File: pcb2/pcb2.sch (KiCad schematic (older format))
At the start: 3 parts

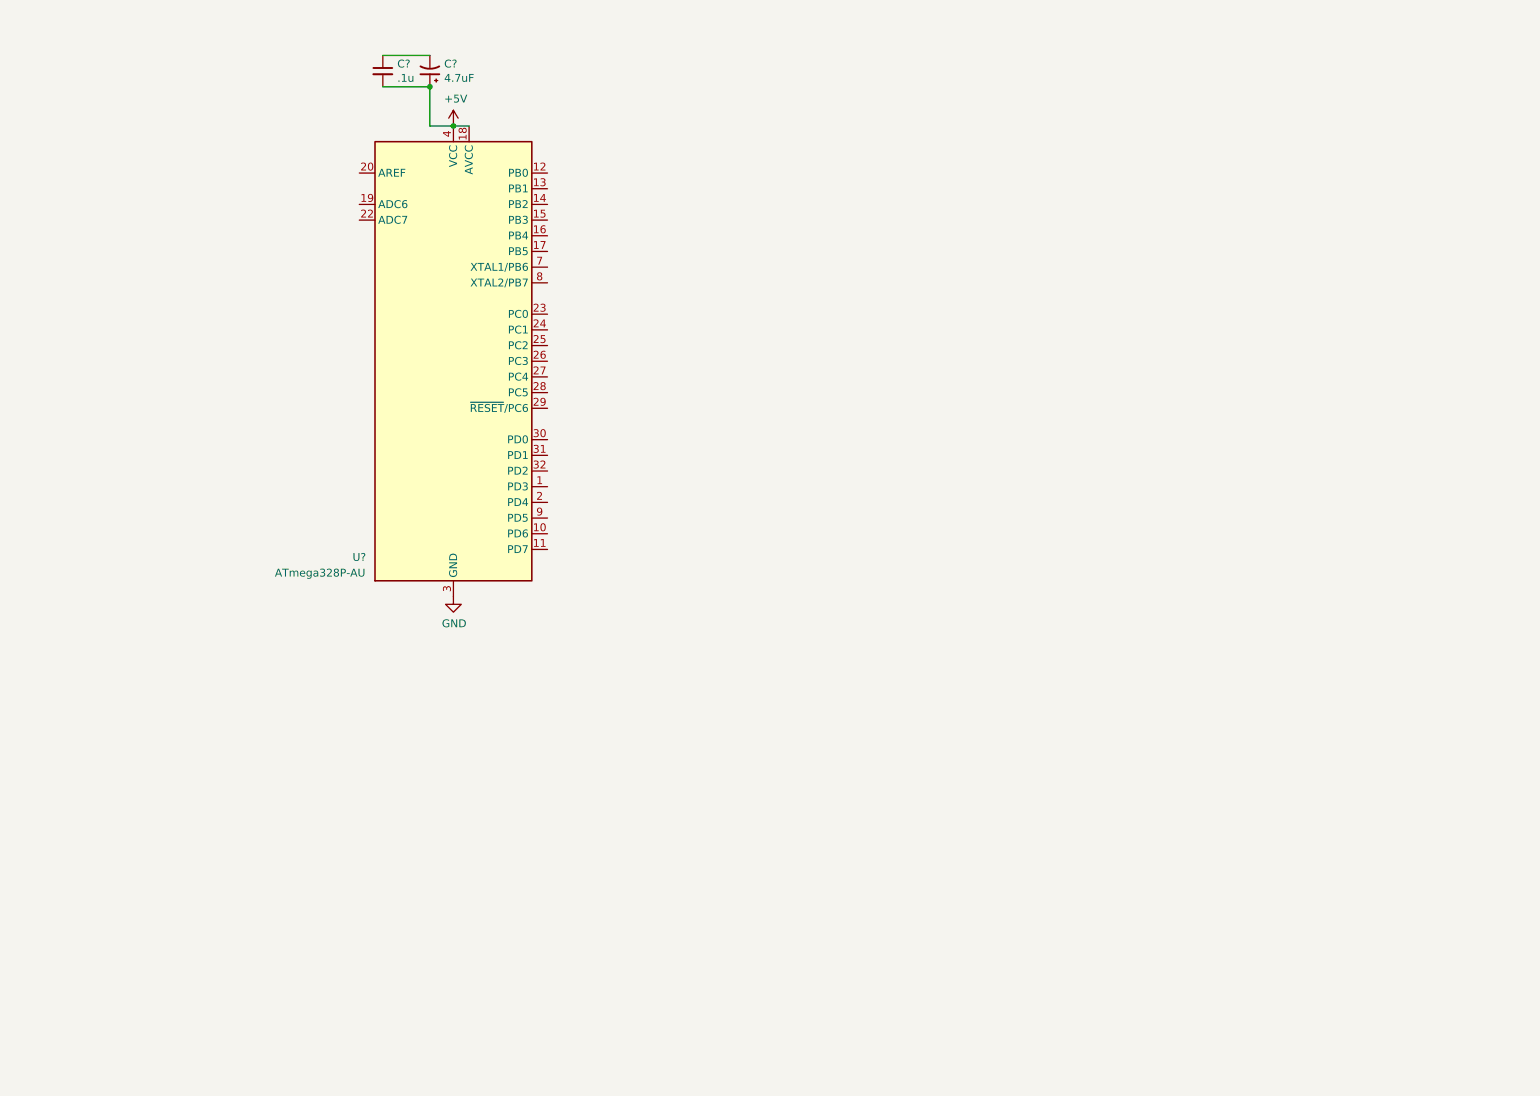
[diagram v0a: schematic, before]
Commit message: second pcb design
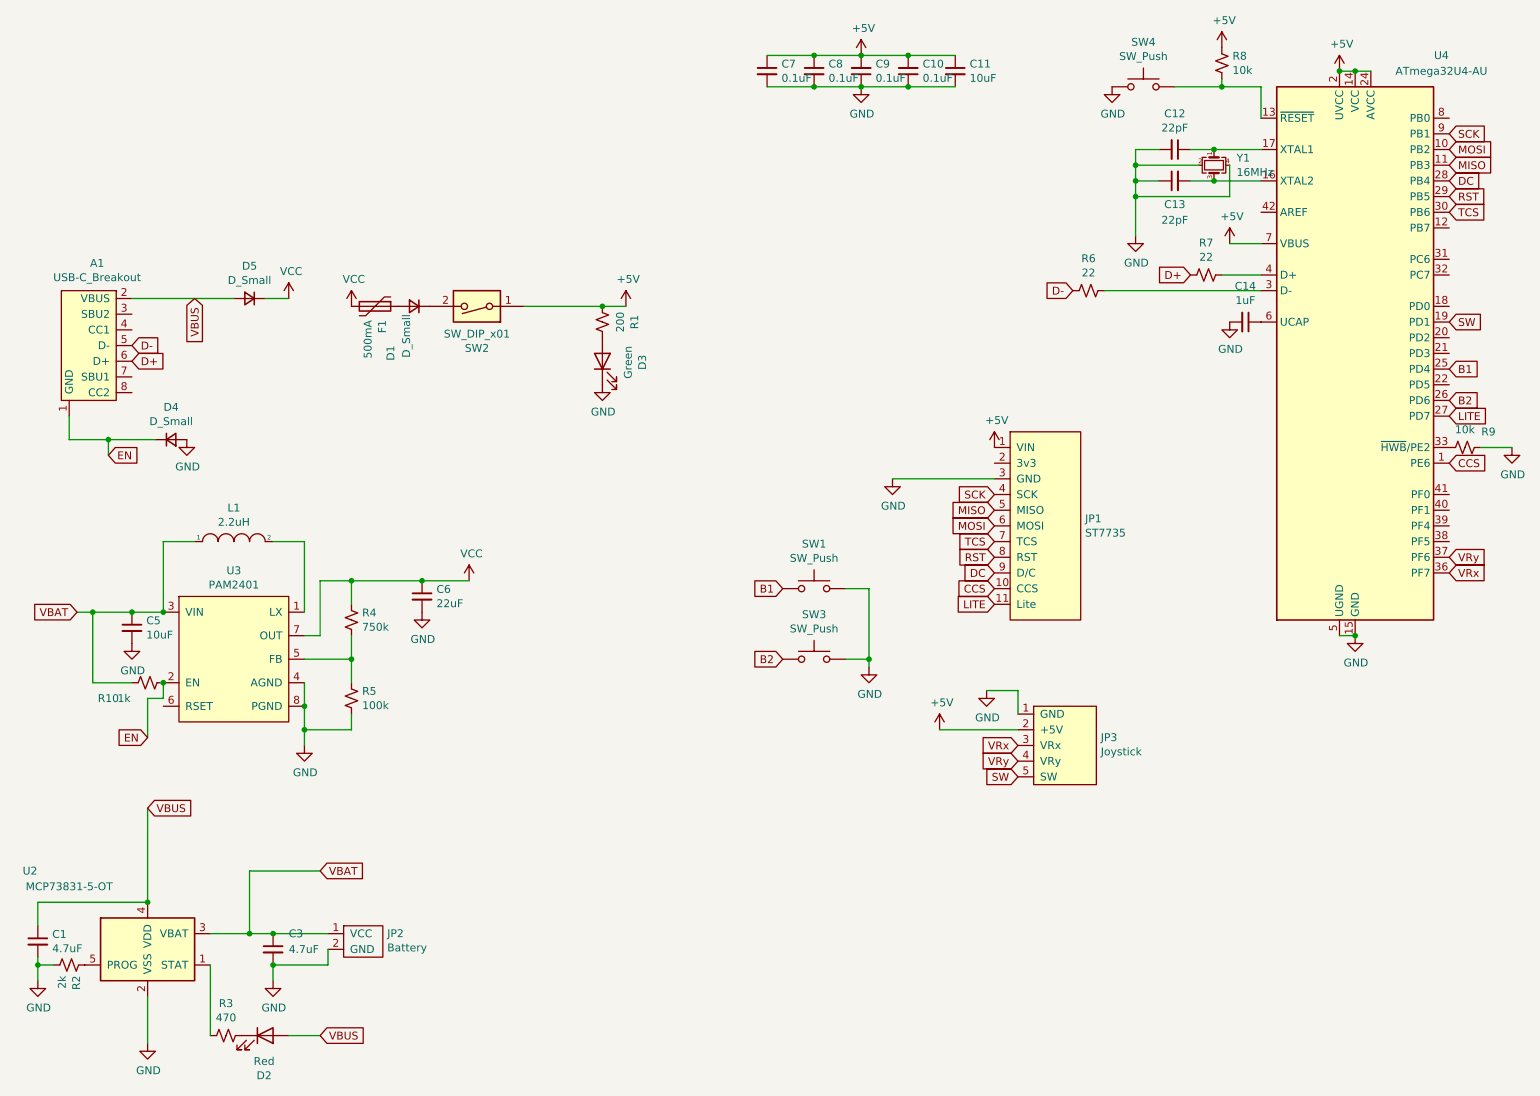
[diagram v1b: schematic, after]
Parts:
- removed C?: .1u, symbol Device:C_Small
- removed C?: 4.7uF, symbol Device:CP1_Small
- removed U?: ATmega328P-AU, Package_QFP:TQFP-32_7x7mm_P0.8mm, symbol MCU_Microchip_ATmega:ATmega328P-AU
- added A1: USB-C_Breakout, pcb2:USB-C_Breakout, symbol pcb2_library:USB-C_Breakout
- added C1, C3: 4.7uF, Capacitor_SMD:C_0805_2012Metric, symbol Device:C_Small
- added C10, C7, C8, C9: 0.1uF, Capacitor_SMD:C_0805_2012Metric, symbol Device:C_Small
- added C11, C5: 10uF, Capacitor_SMD:C_0805_2012Metric, symbol Device:C_Small
- added C12, C13: 22pF, Capacitor_SMD:C_0805_2012Metric, symbol Device:C_Small
- added C14: 1uF, Capacitor_SMD:C_0805_2012Metric, symbol Device:C_Small
- added C6: 22uF, Capacitor_SMD:C_0805_2012Metric, symbol Device:C_Small
- added D1, D4: D_Small, Diode_SMD:D_SOD-123, symbol Device:D_Small
- added D2: Red, LED_SMD:LED_0805_2012Metric, symbol Device:LED
- added D3: Green, LED_SMD:LED_0805_2012Metric, symbol Device:LED
- added D5: D_Small, symbol Device:D_Small
- added F1: 500mA, Fuse:Fuse_1206_3216Metric, symbol Device:Polyfuse
- added JP1: ST7735, pcb2:ST7735, symbol pcb2_library:ST7735
- added JP2: Battery, Connector_PinHeader_2.54mm:PinHeader_1x02_P2.54mm_Vertical, symbol pcb2_library:Battery
- added JP3: Joystick, pcb2:Joystick, symbol pcb2_library:Joystick
- added L1: 2.2uH, Inductor_SMD:L_0805_2012Metric, symbol pspice:INDUCTOR
- added R1: 200, Resistor_SMD:R_0805_2012Metric, symbol Device:R_Small_US
- added R10: 1k, Resistor_SMD:R_0805_2012Metric, symbol Device:R_Small_US
- added R2: 2k, Resistor_SMD:R_0805_2012Metric, symbol Device:R_Small_US
- added R3: 470, Resistor_SMD:R_0805_2012Metric, symbol Device:R_Small_US
- added R4: 750k, Resistor_SMD:R_0805_2012Metric, symbol Device:R_Small_US
- added R5: 100k, Resistor_SMD:R_0805_2012Metric, symbol Device:R_Small_US
- added R6, R7: 22, Resistor_SMD:R_0805_2012Metric, symbol Device:R_Small_US
- added R8, R9: 10k, Resistor_SMD:R_0805_2012Metric, symbol Device:R_Small_US
- added SW1, SW3: SW_Push, pcb2:MX_Switch, symbol Switch:SW_Push
- added SW2: SW_DIP_x01, Connector_PinHeader_2.54mm:PinHeader_1x03_P2.54mm_Vertical, symbol Switch:SW_DIP_x01
- added SW4: SW_Push, Button_Switch_SMD:SW_SPST_SKQG_WithStem, symbol Switch:SW_Push
- added U2: MCP73831-5-OT, Package_TO_SOT_SMD:SOT-23-5, symbol Battery_Management:MCP73831-5-OT
- added U3: PAM2401, Package_SO:MSOP-8_3x3mm_P0.65mm, symbol pcb2_library:PAM2401
- added U4: ATmega32U4-AU, Package_QFP:TQFP-44_10x10mm_P0.8mm, symbol MCU_Microchip_ATmega:ATmega32U4-AU
- added Y1: 16MHz, Crystal:Crystal_SMD_3225-4Pin_3.2x2.5mm, symbol Device:Crystal_GND24_Small
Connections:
- net +5V: now also C10.2, C11.1, C7.1, C8.1, C9.2, JP1.1 (VIN), JP3.2 (+5V), R1.2, R8.1, SW2.1, U4.14 (VCC), U4.2 (UVCC), U4.24 (AVCC), U4.34 (VCC), U4.44 (AVCC), U4.7 (VBUS)
- net GND: now also C1.2, C10.1, C11.2, C12.2, C13.1, C14.2, C3.2, C5.2, C6.2, C7.2, C8.2, C9.1, D3.1 (K), D4.2 (A), JP1.3 (GND), JP2.2 (GND), JP3.1 (GND), R2.2, R5.2, R9.1, SW1.2, SW3.2, SW4.1, U2.2 (VSS), U3.4 (AGND), U3.8 (PGND), U4.15 (GND), U4.23 (GND), U4.35 (GND), U4.43 (GND), U4.5 (UGND), Y1.2, Y1.4
- new net: D1.1 (K), SW2.2
- new net: D1.2 (A), F1.1
- new net: R8.2, SW4.2, U4.13 (~RESET)
- new net: C13.2, U4.16 (XTAL2), Y1.3
- new net: C12.1, U4.17 (XTAL1), Y1.1
- new net: R6.1, U4.3 (D-)
- new net: R9.2, U4.33 (~HWB~/PE2)
- new net: R7.1, U4.4 (D+)
- new net: C14.1, U4.6 (UCAP)
- new net: D3.2 (A), R1.1
- new net: R3.2, U2.1 (STAT)
- new net: R2.1, U2.5 (PROG)
- new net: D2.1 (K), R3.1
- new net: L1.2, U3.1 (LX)
- new net: R4.2, R5.1, U3.5 (FB)
- new net B1: SW1.1, U4.25 (PD4)
- new net B2: SW3.1, U4.26 (PD6)
- new net CCS: JP1.10 (CCS), U4.1 (PE6)
- new net D+: A1.6 (D+), R7.2
- new net D-: A1.5 (D-), R6.2
- new net DC: JP1.9 (D/C), U4.28 (PB4)
- new net EN: A1.1 (GND), D4.1 (K), R10.1, U3.2 (EN)
- new net LITE: JP1.11 (Lite), U4.27 (PD7)
- new net MISO: JP1.5 (MISO), U4.11 (PB3)
- new net MOSI: JP1.6 (MOSI), U4.10 (PB2)
- new net RST: JP1.8 (RST), U4.29 (PB5)
- new net SCK: JP1.4 (SCK), U4.9 (PB1)
- new net SW: JP3.5 (SW), U4.19 (PD1)
- new net TCS: JP1.7 (TCS), U4.30 (PB6)
- new net VBAT: C3.1, C5.1, JP2.1 (VCC), L1.1, R10.2, U2.3 (VBAT), U3.3 (VIN)
- new net VBUS: A1.2 (VBUS), C1.1, D2.2 (A), D5.2 (A), U2.4 (VDD)
- new net VCC: C6.1, D5.1 (K), F1.2, R4.1, U3.7 (OUT)
- new net VRx: JP3.3 (VRx), U4.36 (PF7)
- new net VRy: JP3.4 (VRy), U4.37 (PF6)
